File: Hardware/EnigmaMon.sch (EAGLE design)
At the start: 57 parts, among them IC1 4051N, IC2 TLC5940, IC3 MEGA8-P, T1 BC548, T2 BC548, T3 BC548, T4 BC548, T5 BC548, T6 BC548, T8 BC548, T9 BC548

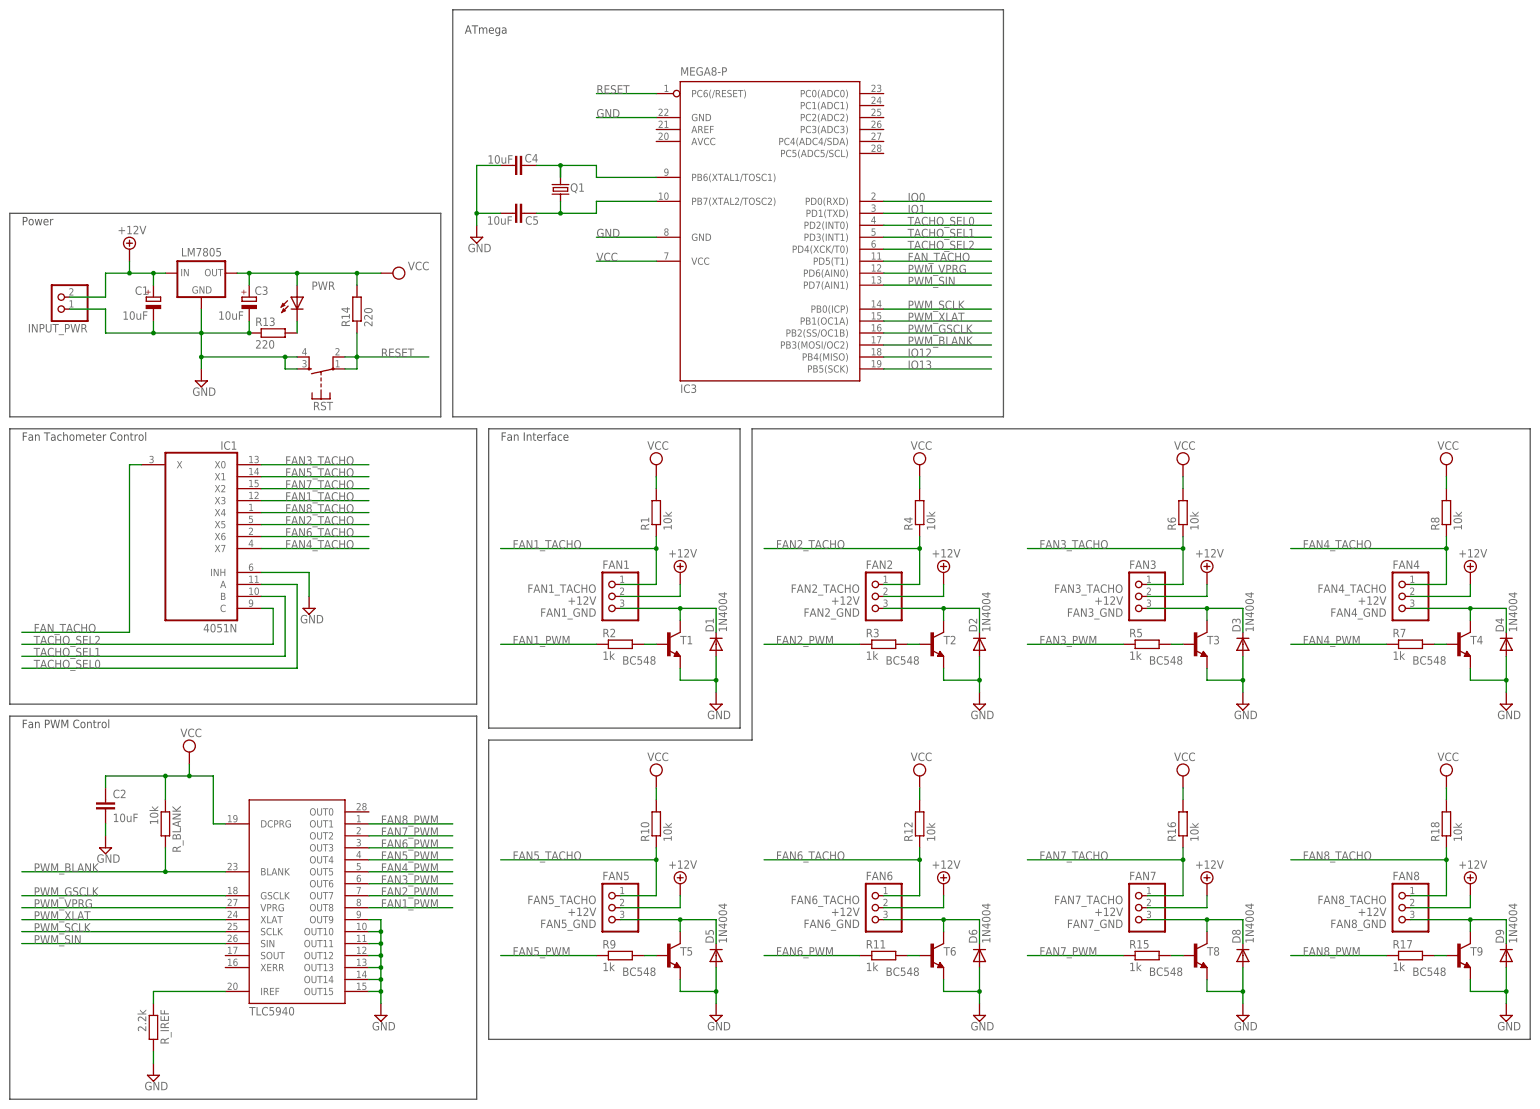
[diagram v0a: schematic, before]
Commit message: Testing
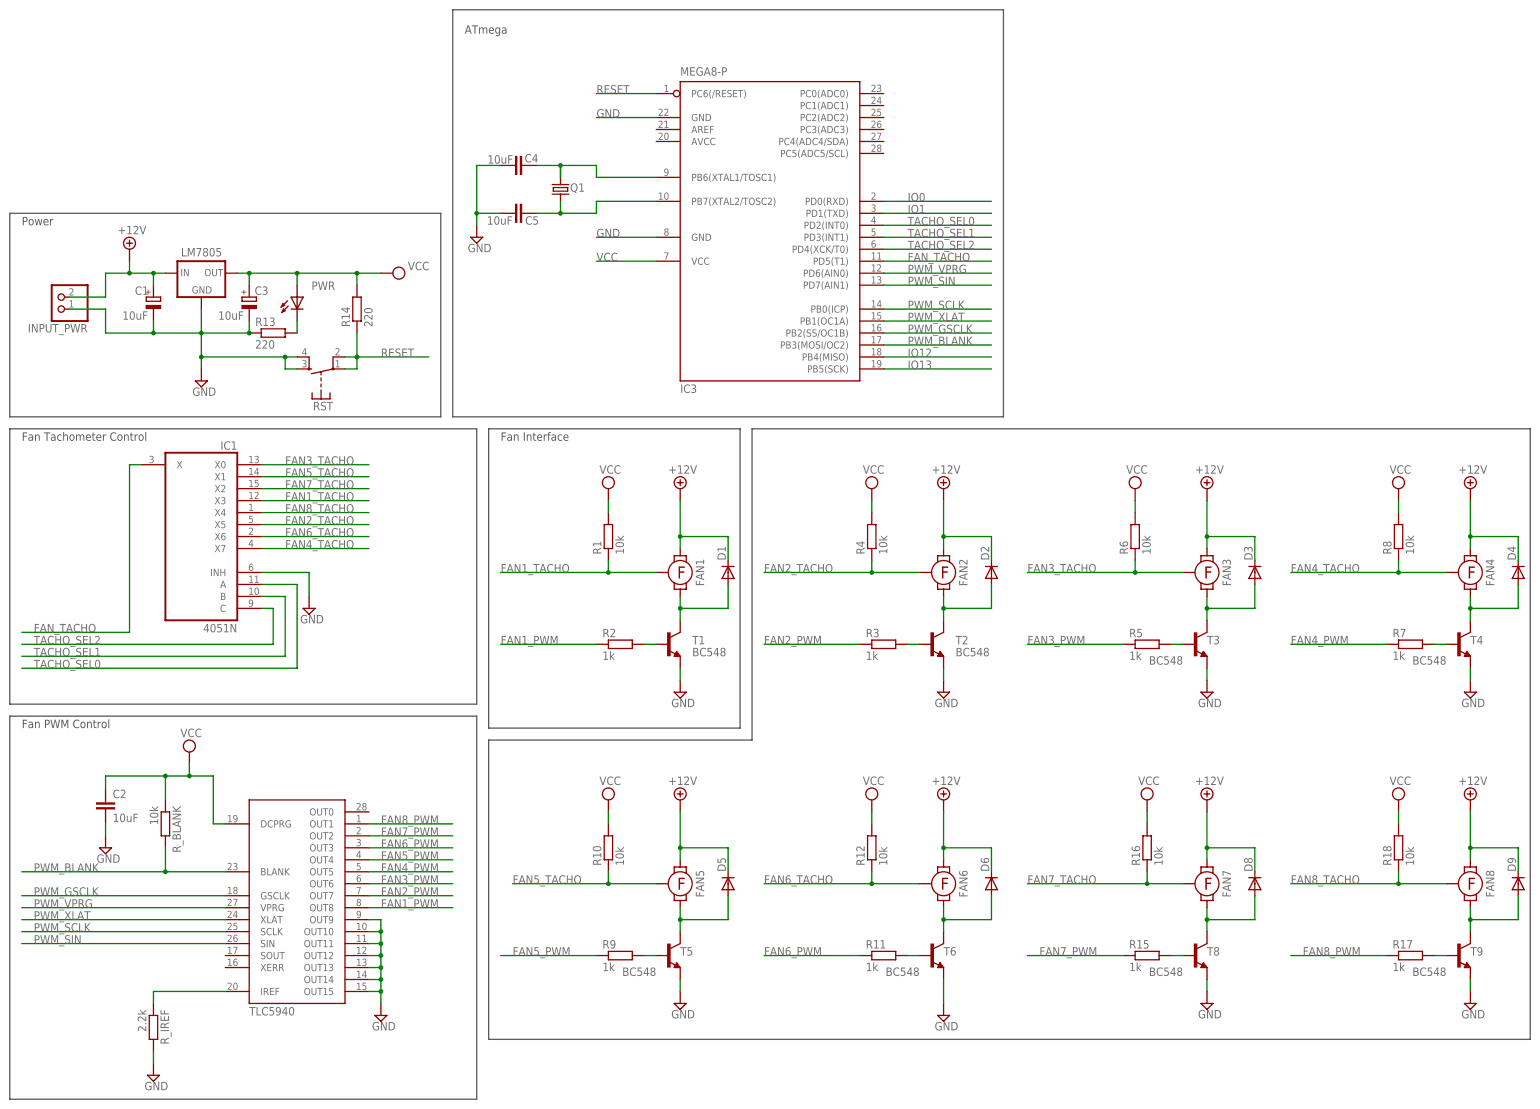
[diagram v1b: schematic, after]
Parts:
- D1, D2, D3, D4, D5, D6, D8, D9: value 1N4004 -> (none); device diode:1N4004 -> diode:DIODE-D-5
- FAN1, FAN2, FAN3, FAN4, FAN5, FAN6, FAN7, FAN8: value (none) -> FAN; device pinhead:PINHD-1X3 -> EnigmaMon:FAN
- R1, R4: device rcl:R-EU_0207/10 -> rcl:R-EU_0204/5
- R10, R11, R12, R15, R16, R17, R18, R2, R3, R5, R6, R7, R8, R9: device rcl:R-EU_0204/7 -> rcl:R-EU_0204/5
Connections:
- removed net FAN1_GND: D1.C, FAN1.3, T1.C
- removed net FAN2_GND: D2.C, FAN2.3, T2.C
- removed net FAN3_GND: D3.C, FAN3.3, T3.C
- removed net FAN4_GND: D4.C, FAN4.3, T4.C
- removed net FAN5_GND: D5.C, FAN5.3, T5.C
- removed net FAN6_GND: D6.C, FAN6.3, T6.C
- removed net FAN7_GND: D8.C, FAN7.3, T8.C
- removed net FAN8_GND: D9.C, FAN8.3, T9.C
- new net N$13: D2.A, FAN2.GND, T2.C
- new net N$14: D3.A, FAN3.GND, T3.C
- new net N$15: D4.A, FAN4.GND, T4.C
- new net N$16: D1.A, FAN1.GND, T1.C
- new net N$17: D9.A, FAN8.GND, T9.C
- new net N$19: D8.A, FAN7.GND, T8.C
- new net N$20: D6.A, FAN6.GND, T6.C
- new net N$21: D5.A, FAN5.GND, T5.C
- net +12V: now also D1.C, D2.C, D3.C, D4.C, D5.C, D6.C, D8.C, D9.C, FAN1.VCC, FAN2.VCC, FAN3.VCC, FAN4.VCC, FAN5.VCC, FAN6.VCC, FAN7.VCC, FAN8.VCC; no longer FAN1.2, FAN2.2, FAN3.2, FAN4.2, FAN5.2, FAN6.2, FAN7.2, FAN8.2
- net FAN1_TACHO: now also FAN1.TACHO; no longer FAN1.1
- net FAN2_TACHO: now also FAN2.TACHO; no longer FAN2.1
- net FAN3_TACHO: now also FAN3.TACHO; no longer FAN3.1
- net FAN4_TACHO: now also FAN4.TACHO; no longer FAN4.1
- net FAN5_TACHO: now also FAN5.TACHO; no longer FAN5.1
- net FAN6_TACHO: now also FAN6.TACHO; no longer FAN6.1
- net FAN7_TACHO: now also FAN7.TACHO; no longer FAN7.1
- net FAN8_TACHO: now also FAN8.TACHO; no longer FAN8.1
- net GND: no longer D1.A, D2.A, D3.A, D4.A, D5.A, D6.A, D8.A, D9.A
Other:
- moved on the sheet: R1, R10, R12, R16, R18, R4, R6, R8
